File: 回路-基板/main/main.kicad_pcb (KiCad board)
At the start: 2 copper layers, 60 x 60 mm, 40 parts, among them J1 Conn_01x07_Pin, SW2 SW_Push, SW3 SW_Push, SW4 SW_Push, SW5 SW_Push, SW6 SW_Push, U1 TWE-L-WX, U2 LM1117MP-3.3

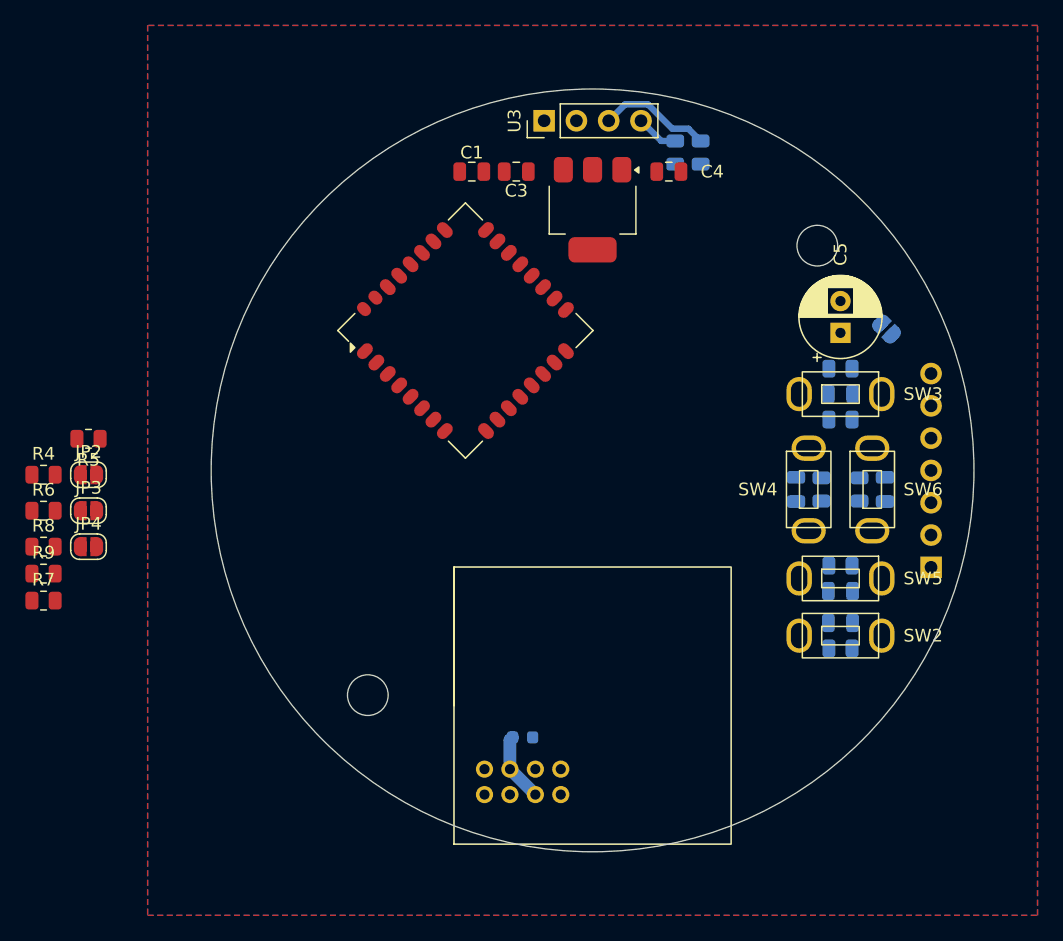
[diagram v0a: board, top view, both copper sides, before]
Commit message: 回路図/PCB両方一応完成した
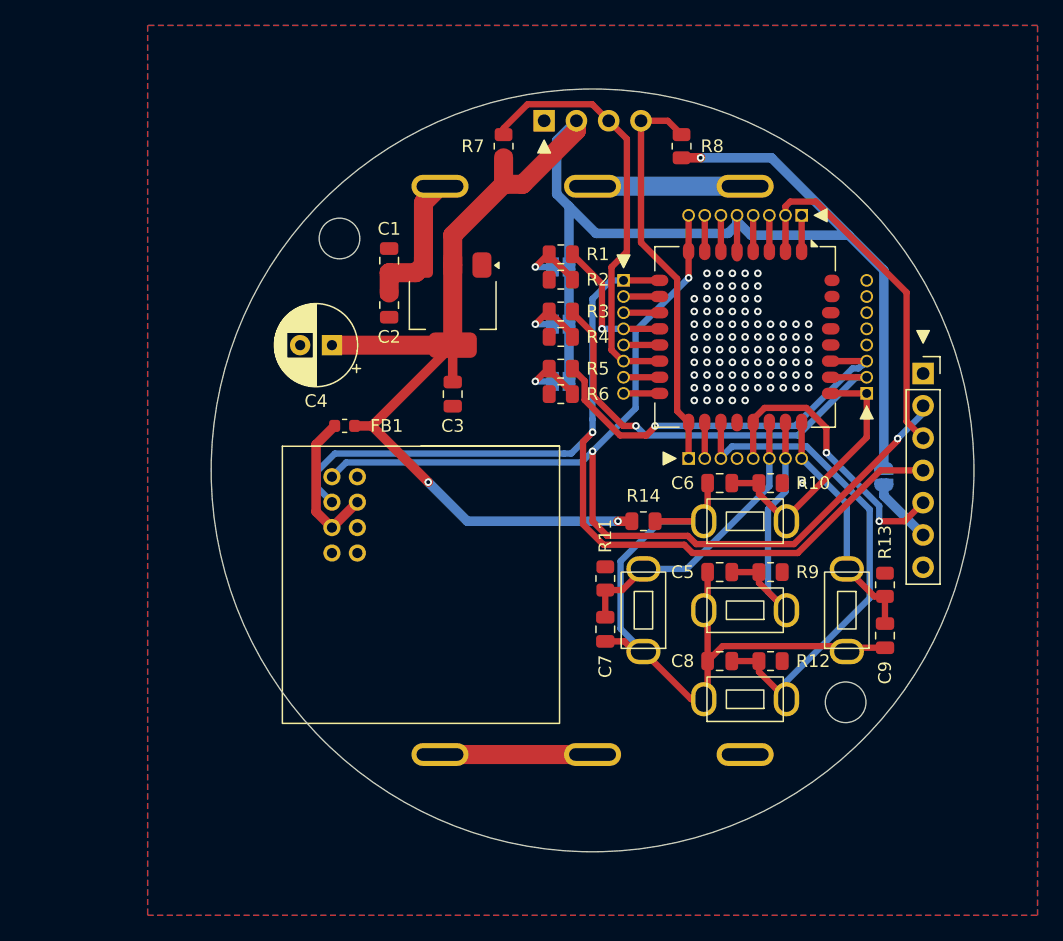
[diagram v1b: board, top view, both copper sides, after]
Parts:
- removed C10: 0.1uF, Capacitor_SMD:C_0805_2012Metric
- removed JP1, JP2, JP3, JP4: Jumper_2_Small_Open, Jumper:SolderJumper-2_P1.3mm_Open_RoundedPad1.0x1.5mm
- removed R15, R16: 100k, Resistor_SMD:R_0805_2012Metric
- removed R17: 10k, Resistor_SMD:R_0805_2012Metric
- removed SW6: SW_Push, @2024-cansat:TVBP06-B043C
- added BT1: 1.5V, @2024-cansat:AAA-holder, B.Cu at (12.0, -22.4)
- added BT2: 1.5V, @2024-cansat:AAA-holder, B.Cu at (0.00, 22.4)
- added BT3: 1.5V, @2024-cansat:AAA-holder, B.Cu at (-12.0, -22.4)
- added C2: 10uF, Capacitor_SMD:C_0805_2012Metric, F.Cu at (-16.0, -13.0)
- added J2: Conn_01x08_Pin, @2024-cansat:Pin-Extender, F.Cu at (16.4, -20.1)
- added J3: Conn_01x08_Pin, @2024-cansat:Pin-Extender, F.Cu at (2.44, -14.9)
- added J4: Conn_01x08_Pin, @2024-cansat:Pin-Extender, F.Cu at (7.55, -0.94)
- added J5: Conn_01x08_Pin, @2024-cansat:Pin-Extender, F.Cu at (21.6, -6.05)
- added M1: Jumper_2_Small_Open, Jumper:SolderJumper-2_P1.3mm_Open_RoundedPad1.0x1.5mm, B.Cu at (-2.50, -16.0)
- added M2: Jumper_2_Small_Open, Jumper:SolderJumper-2_P1.3mm_Open_RoundedPad1.0x1.5mm, B.Cu at (-2.50, -11.5)
- added M3: Jumper_2_Small_Open, Jumper:SolderJumper-2_P1.3mm_Open_RoundedPad1.0x1.5mm, B.Cu at (-2.50, -7.00)
- added R1: 1K, Resistor_SMD:R_0805_2012Metric, F.Cu at (-2.50, -17.0)
- added R2: 10K, Resistor_SMD:R_0805_2012Metric, F.Cu at (-2.50, -15.0)
- added R3: 1K, Resistor_SMD:R_0805_2012Metric, F.Cu at (-2.50, -12.5)
- added SW1: SW_Push, @2024-cansat:TVBP06-B043C, F.Cu at (12.0, 11.0)
- added VBUS/+3.3V: Jumper_2_Small_Open, Jumper:SolderJumper-2_P1.3mm_Open_RoundedPad1.0x1.5mm, B.Cu at (22.9, 0.50)
- C4: value 10uF -> 100uF; footprint Capacitor_SMD:C_0805_2012Metric -> Capacitor_THT:CP_Radial_D6.3mm_P2.50mm
- C5: value 100uF -> 0.1uF; footprint Capacitor_THT:CP_Radial_D6.3mm_P2.50mm -> Capacitor_SMD:C_0805_2012Metric
- C6, C7, C8, C9, FB1, R12, R13: moved to F.Cu
- J1: footprint Connector_PinHeader_2.54mm:PinHeader_1x07_P2.54mm_Horizontal -> Connector_PinSocket_2.54mm:PinSocket_1x07_P2.54mm_Vertical; moved to F.Cu
- R10, R11: value 10K -> 100k; moved to F.Cu
- R14: value 100k -> 10k; moved to F.Cu
- R4, R6, R8: value 1K -> 10K
- R5: value 10K -> 1K
- R9: value 10K -> 100k
- moved R8 59.3 mm to (7.00, -25.5), turned to 90 degrees
- moved R9 57.2 mm to (14.0, 8.00), turned to 180 degrees
- moved R7 50.9 mm to (-7.00, -25.5), turned to 90 degrees
- moved R4 42.1 mm to (-2.50, -10.5)
- moved R6 41.7 mm to (-2.50, -6.00)
- moved REF** 37.6 mm to (19.9, 18.2), turned to 2.5 degrees
- moved REF** 37.6 mm to (-19.9, -18.2), turned to 2.5 degrees
- moved R5 37.6 mm to (-2.50, -8.00)
- moved R11 33.9 mm to (1.00, 8.50), turned to -90 degrees
- moved C4 29.8 mm to (-20.5, -9.85), turned to 180 degrees
- moved FB1 28.2 mm to (-19.5, -3.50)
- moved R10 26.6 mm to (14.0, 1.00), turned to 180 degrees
- moved C7 26.2 mm to (1.00, 12.5), turned to 90 degrees
- moved SW3 23.0 mm to (4.00, 11.0), turned to -90 degrees
- moved U1 22.0 mm to (12.0, -10.5), turned to -90 degrees
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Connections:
- C3 pad 1: VCC -> +3.3V
- C5 pad 1: +3.3V -> Net-(C5-Pad1)
- C5 pad 2: GND -> 23
- C6 pad 1: Net-(C10-Pad1) -> Net-(C5-Pad1)
- C6 pad 2: BTN-CENTER -> 25
- C7 pad 1: Net-(C10-Pad1) -> Net-(C5-Pad1)
- C7 pad 2: BTN-UP -> 22
- C8 pad 1: Net-(C10-Pad1) -> Net-(C5-Pad1)
- C8 pad 2: BTN-LEFT -> 19
- C9 pad 1: Net-(C10-Pad1) -> Net-(C5-Pad1)
- C9 pad 2: BTN-DOWN -> 24
- J1 pad 6: +3.3V -> Net-(J1-Pin_6)
- J1 pad 7: Net-(J1-Pin_7) -> unconnected-(J1-Pin_7-Pad7)
- R10 pad 1: +3.3V -> GND
- R10 pad 2: 14 -> 25
- R11 pad 1: +3.3V -> GND
- R11 pad 2: 17 -> 22
- R12 pad 2: BTN-CENTER -> 19
- R13 pad 2: BTN-UP -> 24
- R14 pad 1: GND -> +3.3V
- R14 pad 2: BTN-LEFT -> Net-(C5-Pad1)
- R4 pad 1: 12 -> GND
- R4 pad 2: Net-(JP2-A) -> Net-(JP3-A)
- R5 pad 1: GND -> 27
- R5 pad 2: Net-(JP2-A) -> Net-(JP4-A)
- R6 pad 1: 26 -> GND
- R6 pad 2: Net-(JP3-A) -> Net-(JP4-A)
- R7 pad 1: GND -> +3.3V
- R7 pad 2: Net-(JP3-A) -> 14
- R8 pad 1: 27 -> +3.3V
- R8 pad 2: Net-(JP4-A) -> 17
- R9 pad 2: Net-(JP4-A) -> 23
- SW2 pad 1: BTN-CENTER -> 25
- SW2 pad 2: Net-(C10-Pad1) -> Net-(C5-Pad1)
- SW3 pad 1: BTN-UP -> 22
- SW3 pad 2: Net-(C10-Pad1) -> Net-(C5-Pad1)
- SW4 pad 1: BTN-LEFT -> 19
- SW4 pad 2: Net-(C10-Pad1) -> Net-(C5-Pad1)
- SW5 pad 1: BTN-DOWN -> 24
- SW5 pad 2: Net-(C10-Pad1) -> Net-(C5-Pad1)
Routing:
- net +3.3V: track 0.00 -> 155.7 mm, vias 0 -> 3
- net 8: track 0.00 -> 80.2 mm, vias 0 -> 3
- net 9: track 0.25 -> 80.1 mm, vias 0 -> 1
- net Net-(C5-Pad1): track 0.00 -> 58.4 mm
- net 19: track 0.00 -> 40.7 mm
- net 26: track 0.00 -> 34.8 mm, vias 0 -> 1
- net 27: track 0.00 -> 31.5 mm, vias 0 -> 1
- net 17: track 3.35 -> 31.8 mm
- net 2: track 0.00 -> 28.2 mm
- net 14: track 9.22 -> 33.4 mm
- net 22: track 0.00 -> 23.4 mm
- net 21: track 0.00 -> 23.0 mm, vias 0 -> 2
- net 23: track 0.00 -> 22.0 mm
- net 25: track 0.00 -> 21.5 mm
- net 24: track 0.00 -> 19.0 mm
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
